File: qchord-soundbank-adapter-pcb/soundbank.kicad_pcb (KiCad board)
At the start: 2 copper layers, 36 x 62 mm, 2 parts, among them U1 8MB ROM, U2 8Mbit Flash

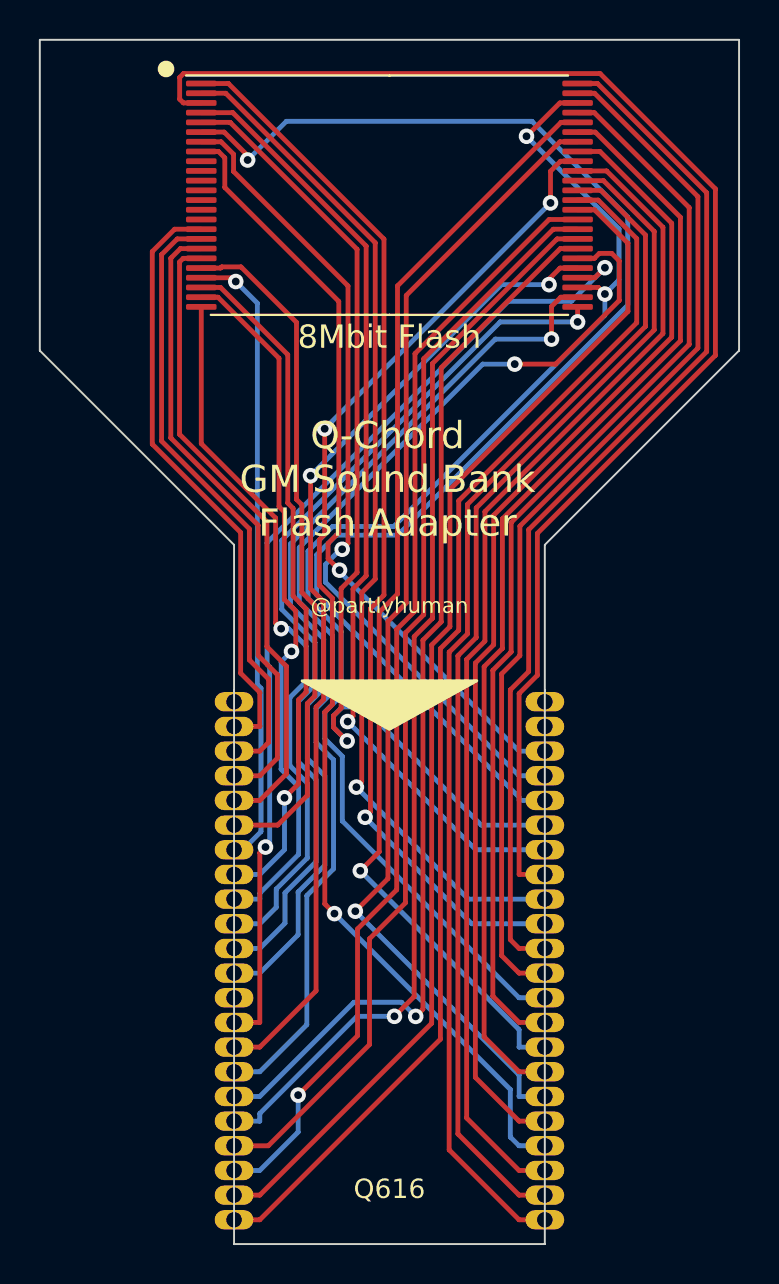
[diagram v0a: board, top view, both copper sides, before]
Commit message: Redesign in-place
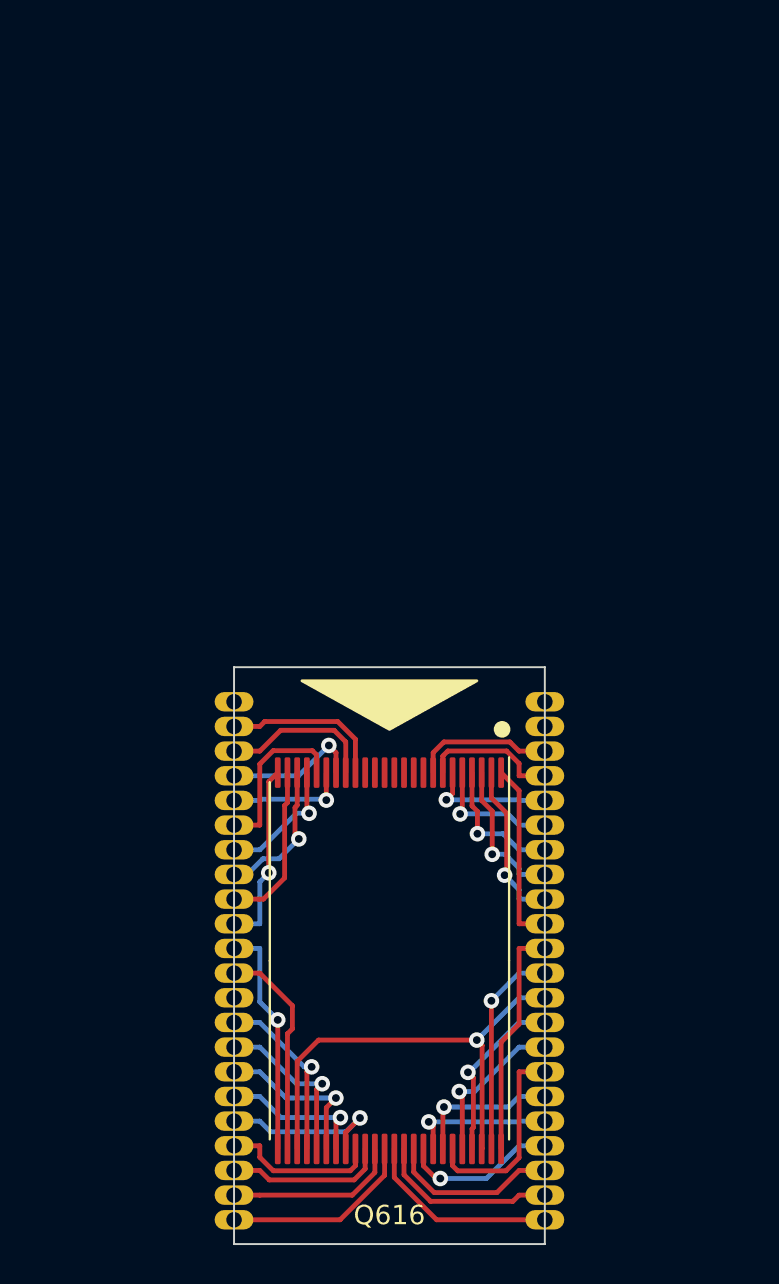
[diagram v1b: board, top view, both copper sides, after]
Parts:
- moved U2 39.4 mm to (94.5, 77.4), turned to -90 degrees
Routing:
- net /A13: track 73.2 -> 7.75 mm, vias 0 -> 1
- net /A10: track 69.7 -> 6.61 mm
- net /Q5: track 62.6 -> 8.09 mm, vias 3 -> 1
- net /Q11: track 63.7 -> 10.1 mm
- net /Q3: track 61.5 -> 8.95 mm
- net /Q4: track 61.5 -> 9.28 mm
- net /VCC: track 62.2 -> 10.1 mm
- net /Q12: track 60.8 -> 8.85 mm
- net /Q6: track 59.2 -> 7.60 mm
- net /Q13: track 59.0 -> 7.48 mm, vias 0 -> 1
- net /Q10: track 57.9 -> 8.22 mm, vias 1 -> 0
- net /Q7: track 57.5 -> 8.38 mm
- net /Q8: track 57.5 -> 8.63 mm
- net /Q2: track 56.3 -> 8.10 mm
- net /Q1: track 55.2 -> 7.63 mm
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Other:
- board size 36 x 62 mm -> 16 x 29.7 mm

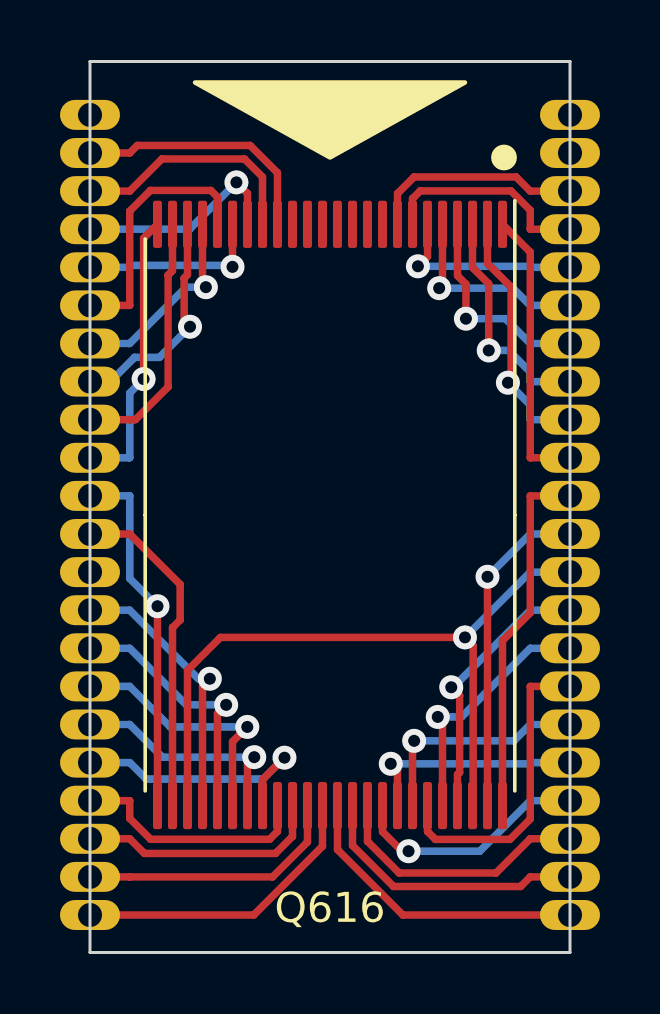
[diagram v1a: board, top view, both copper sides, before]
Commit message: Don't leave stuff floating
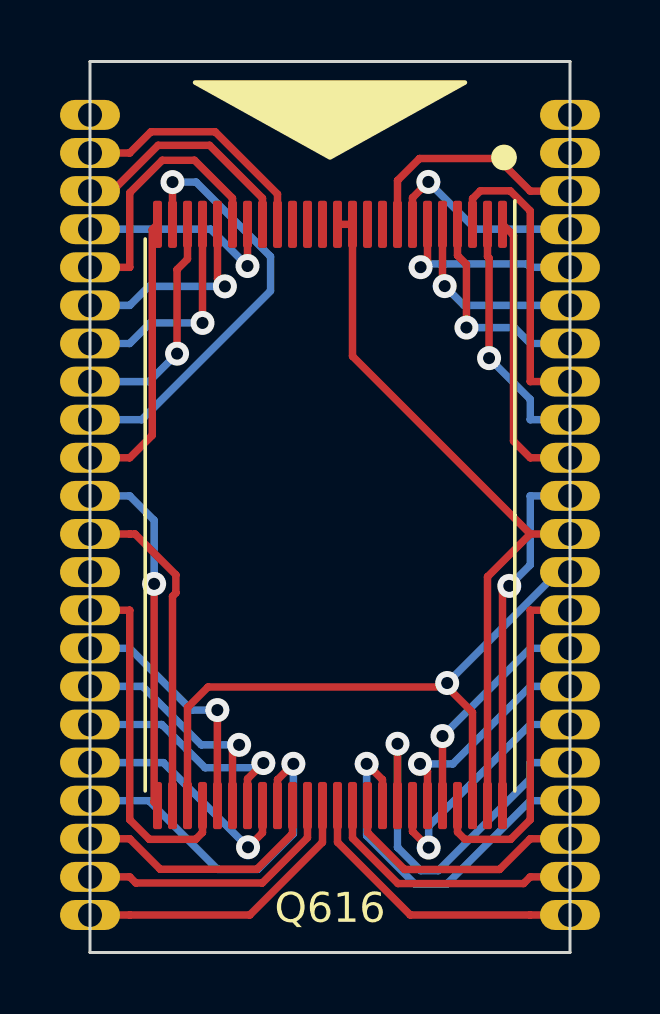
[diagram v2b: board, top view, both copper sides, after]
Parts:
- U1: value 8MB ROM -> 8Mbit ROM
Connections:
- U2 pad 11: unconnected-(U2-~{WE}-Pad11) -> /BYTE
- U2 pad 12: unconnected-(U2-~{RESET}-Pad12) -> /BYTE
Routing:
- net /BYTE: track 11.0 -> 24.2 mm, vias 1 -> 0
- net /A2: track 8.54 -> 14.6 mm, vias 0 -> 1
- net /Q13: track 7.48 -> 13.4 mm
- net /Q5: track 8.09 -> 12.6 mm
- net /Q2: track 8.10 -> 12.2 mm, vias 0 -> 1
- net /Q15: track 9.11 -> 12.0 mm, vias 1 -> 0
- net /A6: track 6.21 -> 9.08 mm, vias 1 -> 0
- net /Q14: track 10.4 -> 7.56 mm, vias 0 -> 1
- net /OE: track 9.27 -> 12.0 mm, vias 1 -> 0
- net /A13: track 7.75 -> 10.2 mm, vias 1 -> 0
- net /GND: track 24.3 -> 22.3 mm
- net /A5: track 8.68 -> 6.93 mm, vias 0 -> 1
- net /Q9: track 8.90 -> 8.03 mm
- net /Q6: track 7.60 -> 8.45 mm
- net /A8: track 7.20 -> 7.96 mm
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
